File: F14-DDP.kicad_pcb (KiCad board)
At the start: 2 copper layers, 106.4 x 65.1 mm, 23 parts, among them SW1 SW_Push, U1 ProMicro

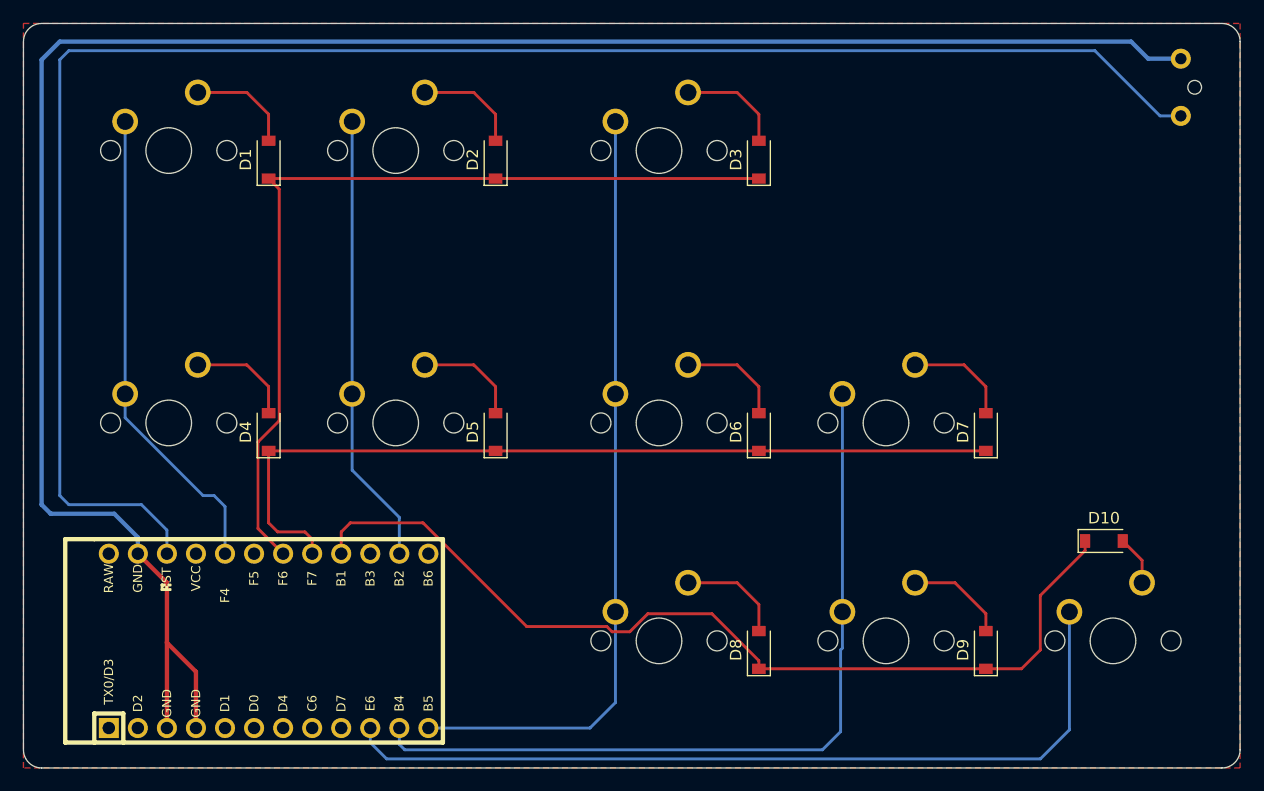
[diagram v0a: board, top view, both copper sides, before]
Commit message: back filling
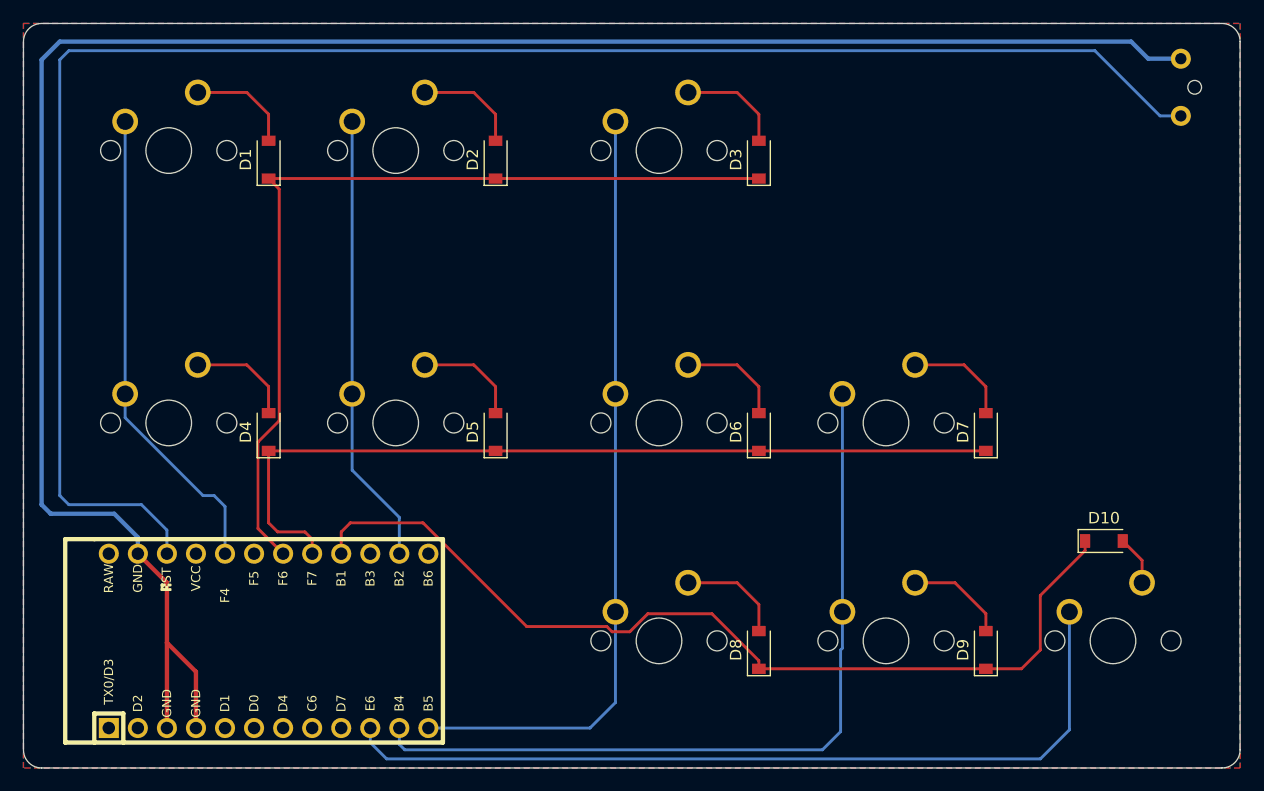
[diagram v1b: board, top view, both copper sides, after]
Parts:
- added G***: LOGO, F14:F14firing, B.Cu at (212.5, 51.8)
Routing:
- added copper zone on B.Cu, net GND
